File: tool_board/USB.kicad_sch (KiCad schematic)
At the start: 2 parts, among them J1 USB_A

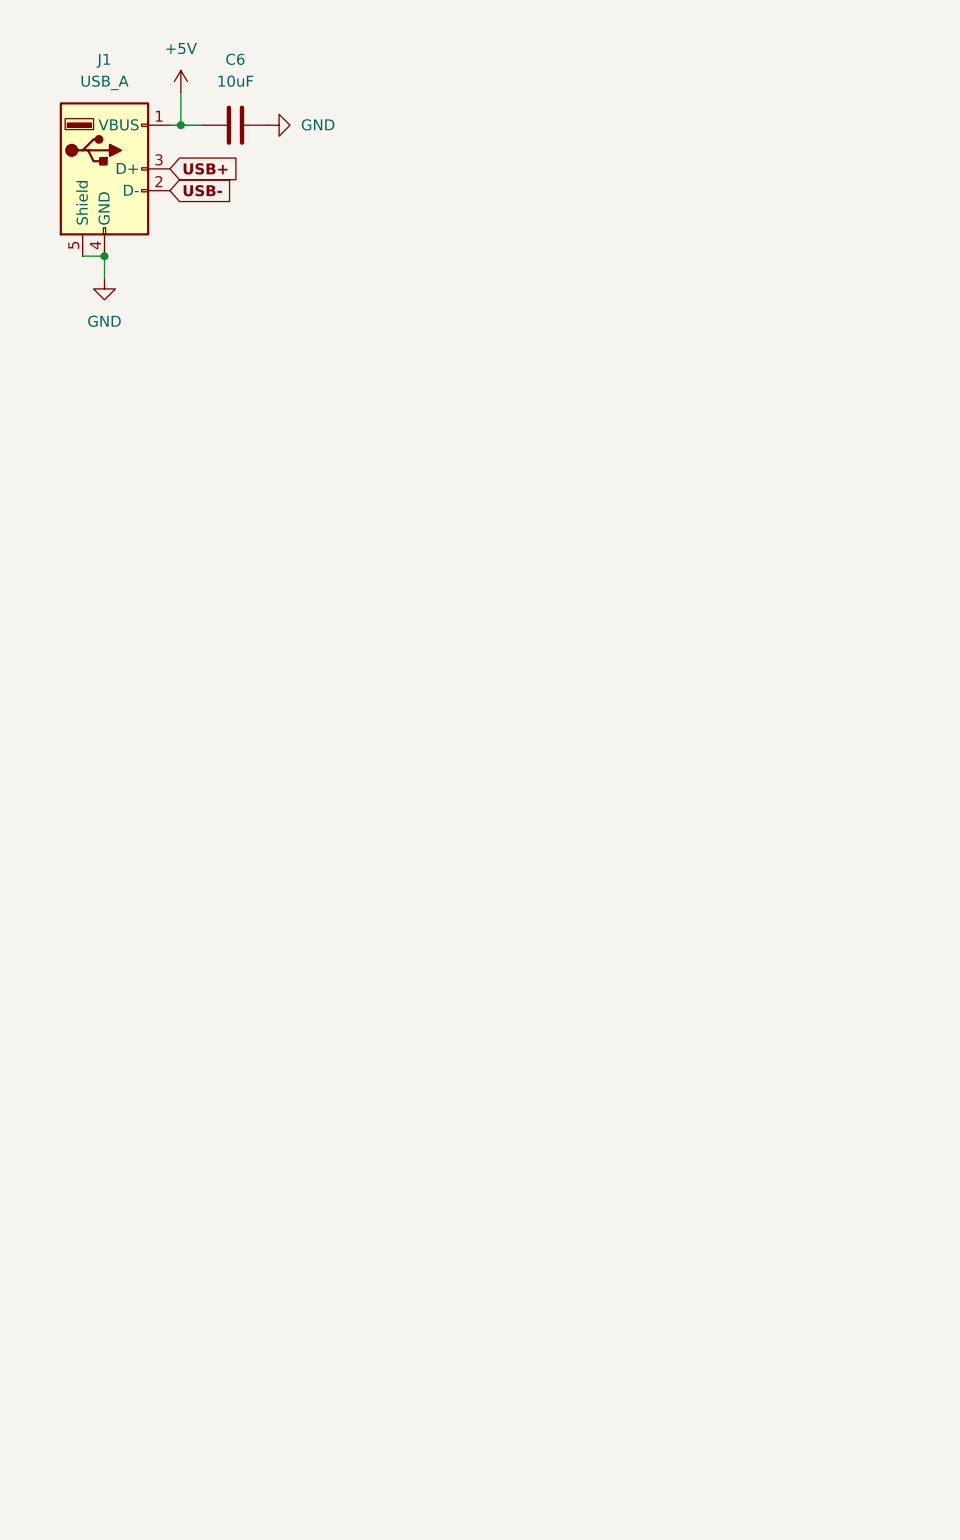
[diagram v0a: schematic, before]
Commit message: message
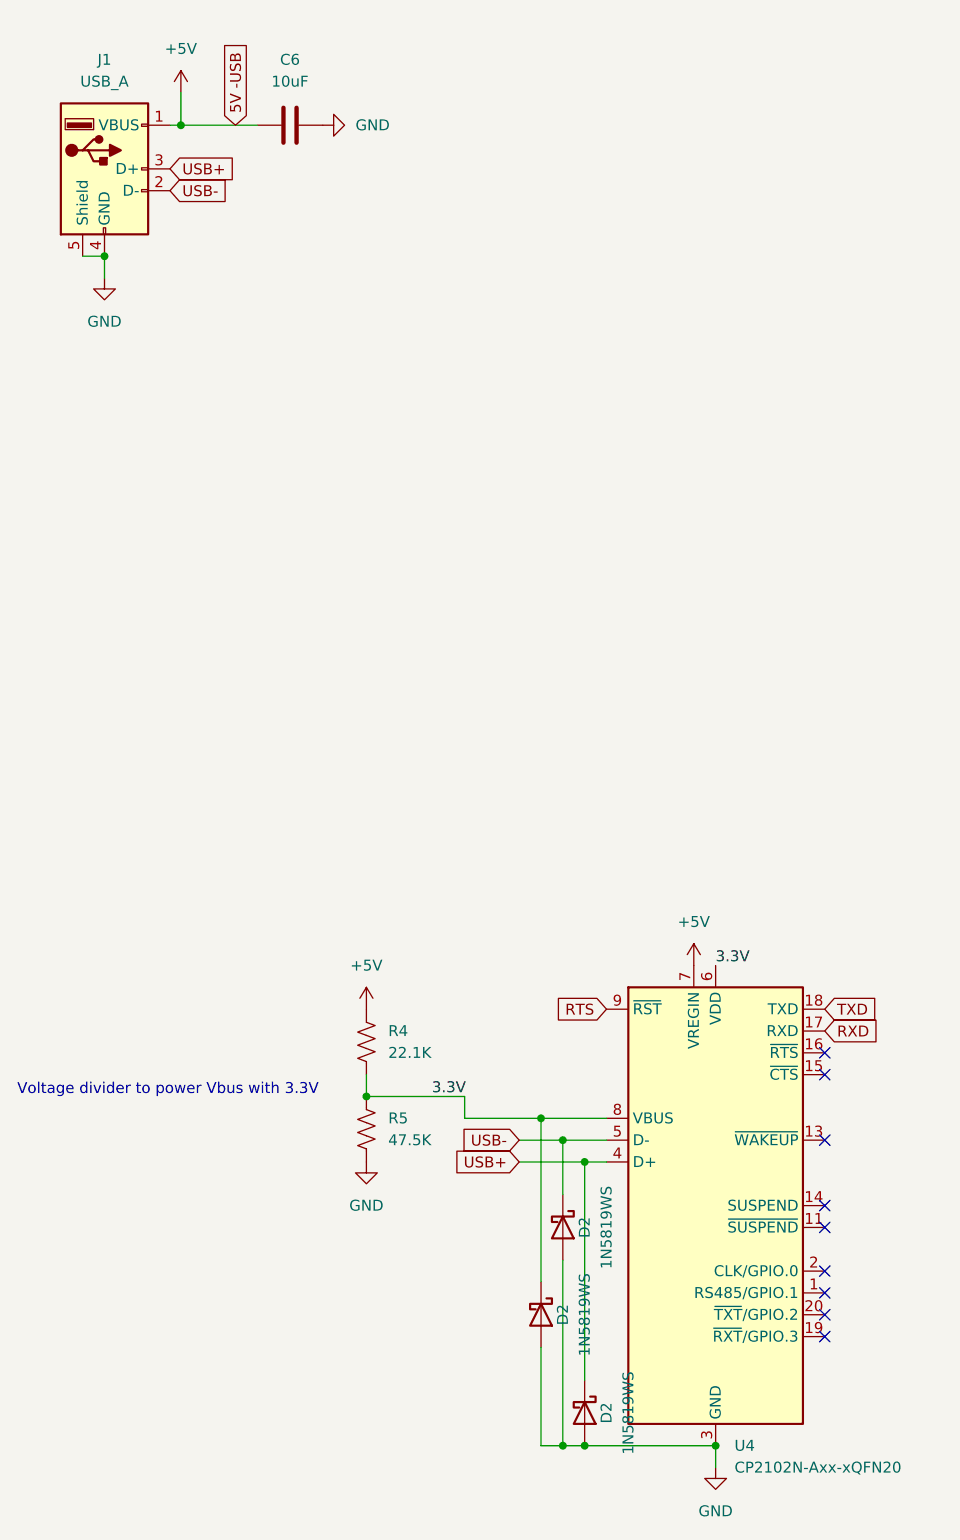
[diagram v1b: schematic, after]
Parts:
- added D2 (x3): 1N5819WS, Diode_SMD:D_SOD-323, symbol Diode:1N5819WS
- added R4: 22.1K, Resistor_SMD:R_0612_1632Metric_Pad1.18x3.40mm_HandSolder, symbol Device:R_US
- added R5: 47.5K, Resistor_SMD:R_0612_1632Metric_Pad1.18x3.40mm_HandSolder, symbol Device:R_US
- added U4: CP2102N-Axx-xQFN20, Package_LGA:LGA-16_3x3mm_P0.5mm_LayoutBorder3x5y, symbol Interface_USB:CP2102N-Axx-xQFN20
- C6: footprint (none) -> Capacitor_SMD:C_0805_2012Metric_Pad1.18x1.45mm_HandSolder
- J1: footprint (none) -> Connector_USB:USB_A_Receptacle_GCT_USB1046
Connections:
- net +5V: now also R4.1, U4.7 (VREGIN)
- net GND: now also D2.2 (A), D2.2 (A), D2.2 (A), R5.2, U4.12 (GND), U4.21 (GND), U4.3 (GND)
- net USB+: now also D2.1 (K), U4.4 (D+)
- net USB-: now also D2.1 (K), U4.5 (D-)
- new net 3.3V: D2.1 (K), R4.2, R5.1, U4.6 (VDD), U4.8 (VBUS)
- new net RTS: U4.9 (~{RST})
- new net RXD: U4.17 (RXD)
- new net TXD: U4.18 (TXD)
- no-connect marks 0 -> 9
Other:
- note added: "Voltage divider to power Vbus with 3.3V"
- moved on the sheet: C6
